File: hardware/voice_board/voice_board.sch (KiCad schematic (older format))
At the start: 114 parts, among them J1 Conn_02x06_Odd_Even, J2 Conn_02x02_Odd_Even, J3 Conn_02x02_Odd_Even, J4 Conn_01x02_Male, J5 Conn_02x03_Odd_Even, Q1 BC327, Q10 BC557, Q11 BC557, Q12 BC557, Q13 BC557, Q14 BC557, Q15 BC557, Q16 BC557, Q17 BC547, Q18 BC547, Q19 2N7000, Q2 BC557, Q20 2N7000, Q3 BC327, Q4 BC557, Q5 BC557, Q6 BC557, Q7 BC557, Q8 BC557, Q9 BC557, U1 TL074, U2 MCP4822

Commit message: rearranged schematic
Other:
- note added: "voltage controlled filter"
- moved on the sheet: C1, C10, C11, C12, C13, C14, C15, C2, C3, C4, C5, C6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

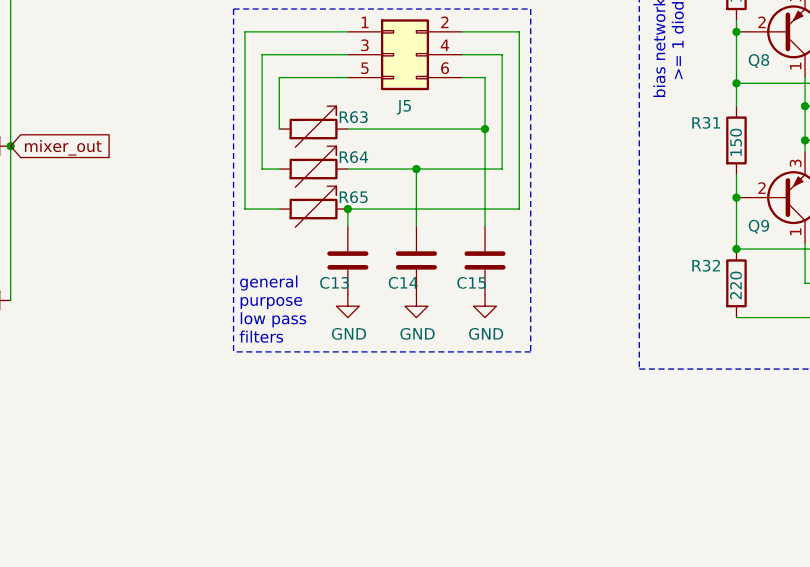
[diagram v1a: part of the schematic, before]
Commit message: voice board: footprint association
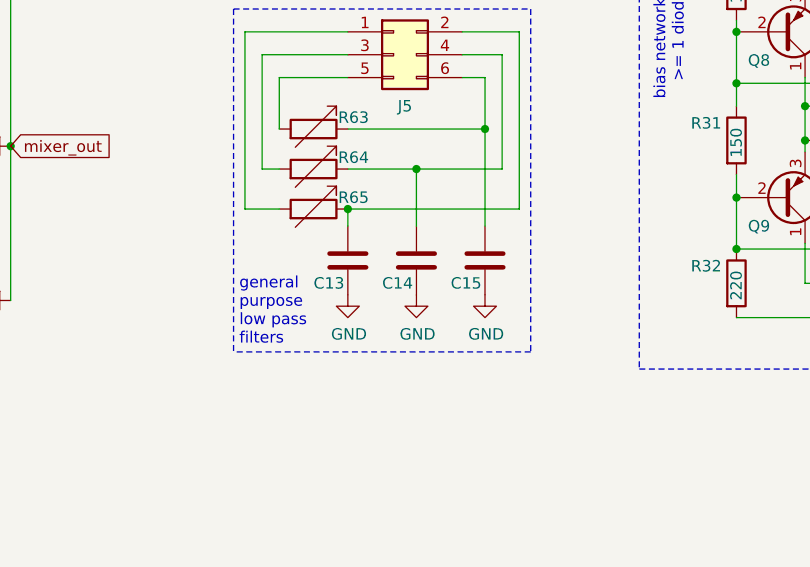
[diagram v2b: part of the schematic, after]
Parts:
- C1, C12, C13, C14, C15, C3, C4, C5, C6, C8, C9: footprint (none) -> Capacitor_SMD:C_0805_2012Metric_Pad1.15x1.40mm_HandSolder
- D1, D2: footprint (none) -> Diode_THT:D_DO-35_SOD27_P7.62mm_Horizontal
- J1: footprint (none) -> Connector_PinHeader_2.54mm:PinHeader_2x06_P2.54mm_Vertical
- J2, J3: footprint (none) -> Connector_PinHeader_2.54mm:PinHeader_2x02_P2.54mm_Vertical
- J4, JP1, JP2: footprint (none) -> Connector_PinHeader_2.54mm:PinHeader_1x02_P2.54mm_Vertical
- J5: footprint (none) -> Connector_PinHeader_2.54mm:PinHeader_2x03_P2.54mm_Vertical
- JP3: footprint (none) -> Connector_PinHeader_2.54mm:PinHeader_1x03_P2.54mm_Vertical
- R1, R18, R19, R2, R20, R52, R53, R54, R55, R57, R58, R59: footprint (none) -> Potentiometer_THT:Potentiometer_Runtron_RM-065_Vertical
- R10, R11, R12, R13, R14, R15, R16, R17, R21, R22, R23, R24, R25, R26, R27, R28, R29, R3, R30, R31, R32, R33, R34, R35, R36, R37, R38, R39, R4, R40, R41, R42, R43, R44, R45, R46, R47, R48, R49, R5, R50, R51, R56, R6, R60, R61, R62, R63, R64, R65, R7, R8, R9: footprint (none) -> Resistor_SMD:R_0805_2012Metric_Pad1.15x1.40mm_HandSolder
- U1: footprint (none) -> Package_DIP:DIP-14_W7.62mm
- U2: footprint (none) -> Package_DIP:DIP-8_W7.62mm

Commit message: more footprints
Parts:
- C10, C11: footprint (none) -> Capacitor_SMD:C_0805_2012Metric_Pad1.15x1.40mm_HandSolder
- C2, C7: footprint (none) -> Capacitor_SMD:CP_Elec_8x5.4
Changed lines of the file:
@@
 F 0 "C2" V 8250 2000 50  0000 C CNN
 F 1 "470u" V 8400 1975 50  0000 C CNN
-F 2 "" H 8363 1975 50  0001 C CNN
+F 2 "Capacitor_SMD:CP_Elec_8x5.4" H 8363 1975 50  0001 C CNN
 F 3 "~" H 8325 2125 50  0001 C CNN
 	1    8325 2125
@@
 F 0 "C7" V 9450 2300 50  0000 C CNN
 F 1 "470u" V 9600 2275 50  0000 C CNN
-F 2 "" H 9563 1975 50  0001 C CNN
+F 2 "Capacitor_SMD:CP_Elec_8x5.4" H 9563 1975 50  0001 C CNN
 F 3 "~" H 9525 2125 50  0001 C CNN
 	1    9525 2125
@@
 F 0 "C10" H 5550 7425 50  0000 L CNN
 F 1 "1u" H 5550 7225 50  0000 L CNN
-F 2 "" H 5713 7175 50  0001 C CNN
+F 2 "Capacitor_SMD:C_0805_2012Metric_Pad1.15x1.40mm_HandSolder" H 5713 7175 50  0001 C CNN
 F 3 "~" H 5675 7325 50  0001 C CNN
 	1    5675 7325
@@
 F 0 "C11" H 5775 7425 50  0000 L CNN
 F 1 "1u" H 5775 7225 50  0000 L CNN
-F 2 "" H 5938 7175 50  0001 C CNN
+F 2 "Capacitor_SMD:C_0805_2012Metric_Pad1.15x1.40mm_HandSolder" H 5938 7175 50  0001 C CNN
 F 3 "~" H 5900 7325 50  0001 C CNN
 	1    5900 7325

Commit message: voice board: fixes, vca layout
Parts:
- R16, R21, R35, R39, R40, R5, R63, R64, R65, R7: footprint Resistor_SMD:R_0805_2012Metric_Pad1.15x1.40mm_HandSolder -> Potentiometer_THT:Potentiometer_Runtron_RM-065_Vertical
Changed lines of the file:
@@
 	2350 1600 2475 1600
-$Comp
-L power:GNDREF #PWR09
-U 1 1 5D95F82A
-P 2775 1800
-F 0 "#PWR09" H 2775 1550 50  0001 C CNN
-F 1 "GNDREF" H 2780 1627 50  0001 C CNN
-F 2 "" H 2775 1800 50  0001 C CNN
-F 3 "" H 2775 1800 50  0001 C CNN
-	1    2775 1800
-	-1   0    0    -1
-$EndComp
 $Comp
 L Transistor_BJT:BC327 Q3
@@
 Text Notes 3100 1550 2    50   ~ 0
 current mirror as\nvoltage controlled\ncurrent source
-$Comp
-L power:GNDREF #PWR05
-U 1 1 5D9C7217
-P 1725 2725
-F 0 "#PWR05" H 1725 2475 50  0001 C CNN
-F 1 "GNDREF" H 1730 2552 50  0001 C CNN
-F 2 "" H 1725 2725 50  0001 C CNN
-F 3 "" H 1725 2725 50  0001 C CNN
-	1    1725 2725
-	1    0    0    -1
-$EndComp
 Text Notes 1650 2750 1    50   ~ 0
 input preattenuation.\ncontrols distortion
@@
 F 0 "R7" H 1775 2275 50  0000 L CNN
 F 1 "100k" H 1775 2200 50  0000 L CNN
-F 2 "Resistor_SMD:R_0805_2012Metric_Pad1.15x1.40mm_HandSolder" V 1655 2275 50  0001 C CNN
+F 2 "Potentiometer_THT:Potentiometer_Runtron_RM-065_Vertical" V 1655 2275 50  0001 C CNN
 F 3 "~" H 1725 2275 50  0001 C CNN
 	1    1725 2275
@@
 F 0 "R21" V 7825 2100 50  0000 L CNN
 F 1 "1Meg" V 7750 1975 50  0000 L CNN
-F 2 "Resistor_SMD:R_0805_2012Metric_Pad1.15x1.40mm_HandSolder" V 7580 2125 50  0001 C CNN
+F 2 "Potentiometer_THT:Potentiometer_Runtron_RM-065_Vertical" V 7580 2125 50  0001 C CNN
 F 3 "~" H 7650 2125 50  0001 C CNN
 	1    7650 2125
@@
 F 0 "R35" V 9425 2250 50  0000 L CNN
 F 1 "470" V 9525 2250 50  0000 L CNN
-F 2 "Resistor_SMD:R_0805_2012Metric_Pad1.15x1.40mm_HandSolder" V 9455 2325 50  0001 C CNN
+F 2 "Potentiometer_THT:Potentiometer_Runtron_RM-065_Vertical" V 9455 2325 50  0001 C CNN
 F 3 "~" H 9525 2325 50  0001 C CNN
 	1    9525 2325
@@
 F 0 "R40" H 10028 2321 50  0000 L CNN
 F 1 "100k" H 9975 2225 50  0000 L CNN
-F 2 "Resistor_SMD:R_0805_2012Metric_Pad1.15x1.40mm_HandSolder" V 9830 2275 50  0001 C CNN
+F 2 "Potentiometer_THT:Potentiometer_Runtron_RM-065_Vertical" V 9830 2275 50  0001 C CNN
 F 3 "~" H 9900 2275 50  0001 C CNN
 	1    9900 2275
@@
 F 0 "R39" H 9925 1525 50  0000 L CNN
 F 1 "10k" H 9925 1450 50  0000 L CNN
-F 2 "Resistor_SMD:R_0805_2012Metric_Pad1.15x1.40mm_HandSolder" V 9805 1525 50  0001 C CNN
+F 2 "Potentiometer_THT:Potentiometer_Runtron_RM-065_Vertical" V 9805 1525 50  0001 C CNN
 F 3 "~" H 9875 1525 50  0001 C CNN
 	1    9875 1525
@@
 F 0 "R16" H 3350 1100 50  0000 L CNN
 F 1 "100k" H 3350 1025 50  0000 L CNN
-F 2 "Resistor_SMD:R_0805_2012Metric_Pad1.15x1.40mm_HandSolder" V 3230 1100 50  0001 C CNN
+F 2 "Potentiometer_THT:Potentiometer_Runtron_RM-065_Vertical" V 3230 1100 50  0001 C CNN
 F 3 "~" H 3300 1100 50  0001 C CNN
 	1    3300 1100
@@
 F 0 "R5" V 1175 950 50  0000 C CNN
 F 1 "200k" V 1175 1125 50  0000 C CNN
-F 2 "Resistor_SMD:R_0805_2012Metric_Pad1.15x1.40mm_HandSolder" V 1205 1075 50  0001 C CNN
+F 2 "Potentiometer_THT:Potentiometer_Runtron_RM-065_Vertical" V 1205 1075 50  0001 C CNN
 F 3 "~" H 1275 1075 50  0001 C CNN
 	1    1275 1075
@@
 F 0 "R65" V 6675 5050 50  0000 C CNN
 F 1 "any" V 6500 4800 50  0001 C CNN
-F 2 "Resistor_SMD:R_0805_2012Metric_Pad1.15x1.40mm_HandSolder" V 6555 4875 50  0001 C CNN
+F 2 "Potentiometer_THT:Potentiometer_Runtron_RM-065_Vertical" V 6555 4875 50  0001 C CNN
 F 3 "~" H 6625 4875 50  0001 C CNN
 	1    6625 4875
@@
 F 0 "R64" V 6675 4875 50  0000 C CNN
 F 1 "any" V 6500 4625 50  0001 C CNN
-F 2 "Resistor_SMD:R_0805_2012Metric_Pad1.15x1.40mm_HandSolder" V 6555 4700 50  0001 C CNN
+F 2 "Potentiometer_THT:Potentiometer_Runtron_RM-065_Vertical" V 6555 4700 50  0001 C CNN
 F 3 "~" H 6625 4700 50  0001 C CNN
 	1    6625 4700
@@
 F 0 "R63" V 6675 4700 50  0000 C CNN
 F 1 "any" V 6500 4450 50  0001 C CNN
-F 2 "Resistor_SMD:R_0805_2012Metric_Pad1.15x1.40mm_HandSolder" V 6555 4525 50  0001 C CNN
+F 2 "Potentiometer_THT:Potentiometer_Runtron_RM-065_Vertical" V 6555 4525 50  0001 C CNN
 F 3 "~" H 6625 4525 50  0001 C CNN
 	1    6625 4525
@@
 Text Notes 10225 5550 0    50   ~ 0
 voltage controlled filter
+$Comp
+L power:GND #PWR0101
+U 1 1 5DEAC77F
+P 2775 1800
+F 0 "#PWR0101" H 2775 1550 50  0001 C CNN
+F 1 "GND" H 2775 1650 50  0001 C CNN
+F 2 "" H 2775 1800 50  0001 C CNN
+F 3 "" H 2775 1800 50  0001 C CNN
+	1    2775 1800
+	-1   0    0    -1
+$EndComp
+$Comp
+L power:GND #PWR?
+U 1 1 5DEDEEFF
+P 1725 2725
+F 0 "#PWR?" H 1725 2475 50  0001 C CNN
+F 1 "GND" H 1725 2575 50  0001 C CNN
+F 2 "" H 1725 2725 50  0001 C CNN
+F 3 "" H 1725 2725 50  0001 C CNN
+	1    1725 2725
+	-1   0    0    -1
+$EndComp
 $EndSCHEMATC

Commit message: voice board: vcf
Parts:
- R35: footprint Potentiometer_THT:Potentiometer_Runtron_RM-065_Vertical -> Resistor_SMD:R_0805_2012Metric_Pad1.15x1.40mm_HandSolder
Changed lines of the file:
@@
 F 0 "R35" V 9425 2250 50  0000 L CNN
 F 1 "470" V 9525 2250 50  0000 L CNN
-F 2 "Potentiometer_THT:Potentiometer_Runtron_RM-065_Vertical" V 9455 2325 50  0001 C CNN
+F 2 "Resistor_SMD:R_0805_2012Metric_Pad1.15x1.40mm_HandSolder" V 9455 2325 50  0001 C CNN
 F 3 "~" H 9525 2325 50  0001 C CNN
 	1    9525 2325
@@
 $EndComp
 $Comp
-L power:GND #PWR?
+L power:GND #PWR0102
 U 1 1 5DEDEEFF
 P 1725 2725
-F 0 "#PWR?" H 1725 2475 50  0001 C CNN
+F 0 "#PWR0102" H 1725 2475 50  0001 C CNN
 F 1 "GND" H 1725 2575 50  0001 C CNN
 F 2 "" H 1725 2725 50  0001 C CNN

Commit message: mixer and lowpass filters
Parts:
- added J6: Conn_02x02_Odd_Even, Connector_PinHeader_2.54mm:PinHeader_2x02_P2.54mm_Vertical, symbol Connector_Generic:Conn_02x02_Odd_Even
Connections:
- net labels removed: GNDREF
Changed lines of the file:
@@
 Wire Wire Line
 	1725 1825 1425 1825
-$Comp
-L power:GNDREF #PWR016
-U 1 1 5DC870C2
-P 7800 2425
-F 0 "#PWR016" H 7800 2175 50  0001 C CNN
-F 1 "GNDREF" H 7805 2252 50  0001 C CNN
-F 2 "" H 7800 2425 50  0001 C CNN
-F 3 "" H 7800 2425 50  0001 C CNN
-	1    7800 2425
-	1    0    0    -1
-$EndComp
 Text Notes 7675 2975 1    50   ~ 0
 input preattenuation.\ncontrols distortion
@@
 	-1   0    0    -1
 $EndComp
+$Comp
+L power:GND #PWR05
+U 1 1 5DFD1A89
+P 7800 2425
+F 0 "#PWR05" H 7800 2175 50  0001 C CNN
+F 1 "GND" H 7805 2252 50  0001 C CNN
+F 2 "" H 7800 2425 50  0001 C CNN
+F 3 "" H 7800 2425 50  0001 C CNN
+	1    7800 2425
+	-1   0    0    -1
+$EndComp
+$Comp
+L Connector_Generic:Conn_02x02_Odd_Even J6
+U 1 1 5DD854EC
+P 4775 5850
+F 0 "J6" H 4825 5975 50  0000 C CNN
+F 1 "Conn_02x02_Odd_Even" H 4825 5976 50  0001 C CNN
+F 2 "Connector_PinHeader_2.54mm:PinHeader_2x02_P2.54mm_Vertical" H 4775 5850 50  0001 C CNN
+F 3 "~" H 4775 5850 50  0001 C CNN
+	1    4775 5850
+	1    0    0    -1
+$EndComp
+Text GLabel 4575 5850 0    50   Input ~ 0
+vco1_in
+Text GLabel 4575 5950 0    50   Input ~ 0
+vco2_in
+Text GLabel 5075 5850 2    50   Input ~ 0
+vco3_in
+Text GLabel 5075 5950 2    50   Input ~ 0
+mixer_out
 $EndSCHEMATC
